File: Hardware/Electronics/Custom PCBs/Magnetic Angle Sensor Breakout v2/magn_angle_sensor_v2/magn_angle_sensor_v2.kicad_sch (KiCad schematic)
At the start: 57 parts, among them J1 JST PH 01x04, J2 USB C Receptacle, J3 120TR, U1 MT6701-CT, U2 RP2040, U2 W25Q128JVS, U4 SE8650X2-HF, U5 SN65HVD1050D, U6 XC6206P332MR, Y1 12MHz/12pF/50Ω/20ppm

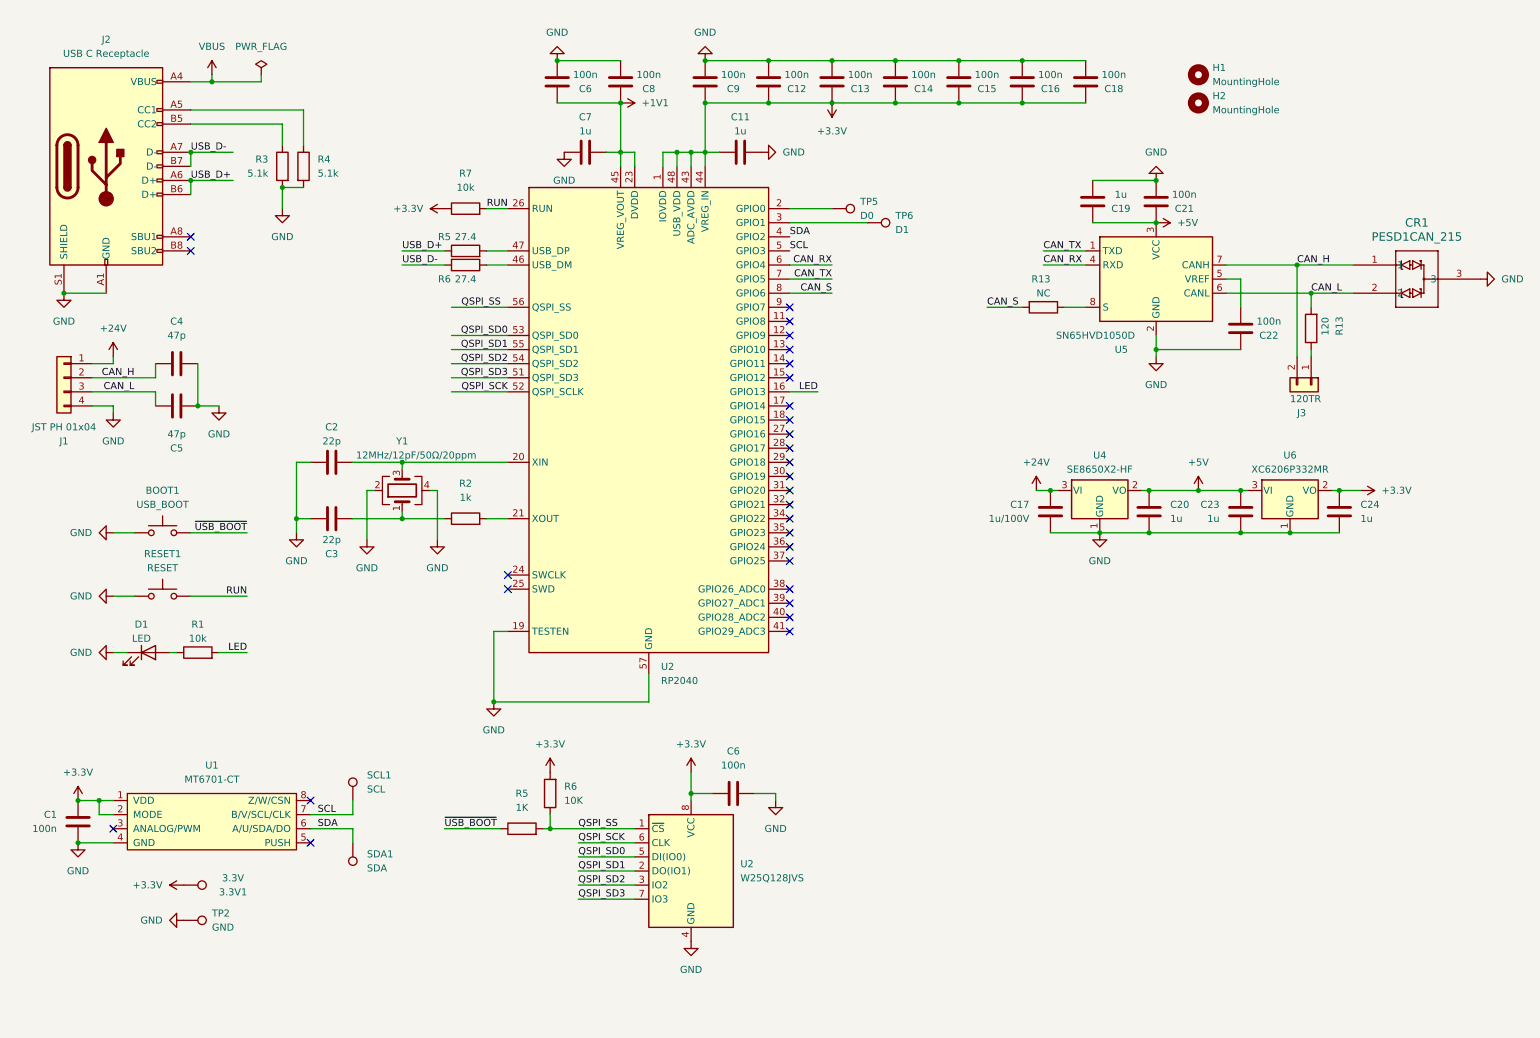
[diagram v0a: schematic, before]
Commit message: Finish CAN Magnetic Angle Sensor v2
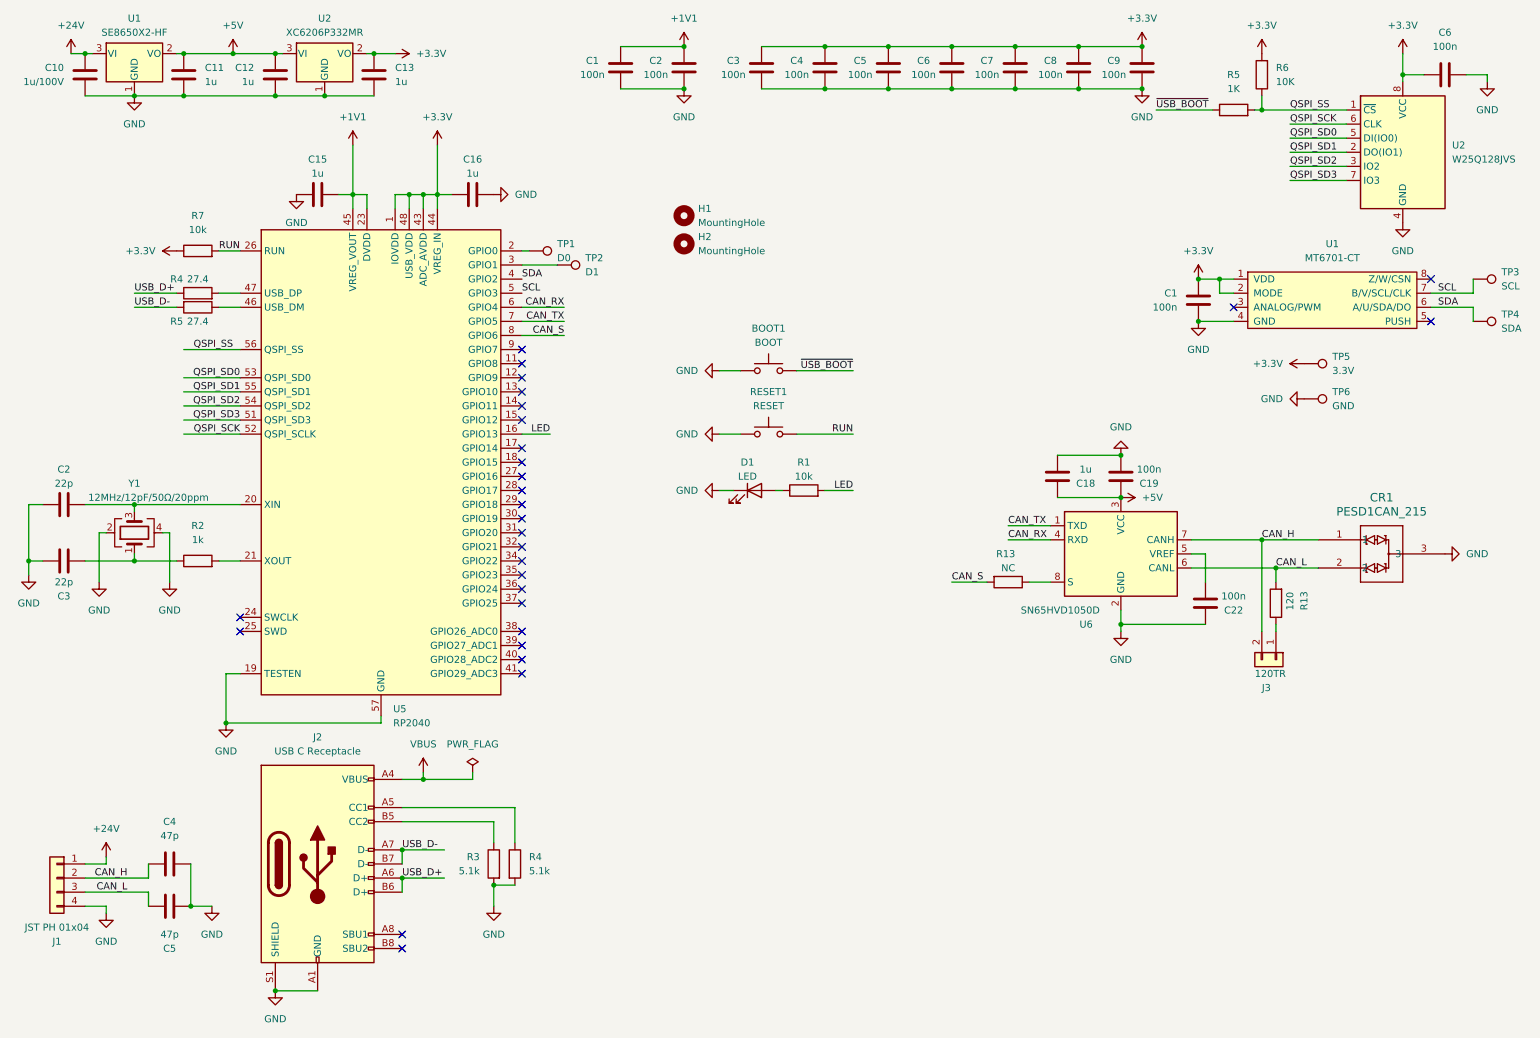
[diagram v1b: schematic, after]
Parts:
- removed 3.3V1: 3.3V, TestPoint:TestPoint_Pad_D1.0mm, symbol Connector:TestPoint
- removed C1, C14, C21, C6 (x2): 100n, Capacitor_SMD:C_0402_1005Metric, symbol Device:C
- removed C17: 1u/100V, Capacitor_SMD:C_0805_2012Metric, symbol Device:C
- removed C2, C3: 22p, Capacitor_SMD:C_0402_1005Metric, symbol Device:C
- removed C20, C23, C24: 1u, Capacitor_SMD:C_0402_1005Metric, symbol Device:C
- removed C4, C5: 47p, Capacitor_SMD:C_0402_1005Metric, symbol Device:C
- removed R13: 120, Resistor_SMD:R_0402_1005Metric, symbol Device:R
- removed R13: NC, Resistor_SMD:R_0402_1005Metric, symbol Device:R
- removed R4: 5.1k, Resistor_SMD:R_0402_1005Metric, symbol Device:R
- removed R5, R6: 27.4, Resistor_SMD:R_0402_1005Metric, symbol Device:R
- removed R5: 1K, Resistor_SMD:R_0402_1005Metric, symbol Device:R
- removed R6: 10K, Resistor_SMD:R_0402_1005Metric, symbol Device:R
- removed SCL1: SCL, TestPoint:TestPoint_Pad_D1.0mm, symbol Connector:TestPoint
- removed SDA1: SDA, TestPoint:TestPoint_Pad_D1.0mm, symbol Connector:TestPoint
- removed U2: RP2040, Package_DFN_QFN:QFN-56-1EP_7x7mm_P0.4mm_EP3.2x3.2mm, symbol MCU_RaspberryPi:RP2040
- removed U4: SE8650X2-HF, Package_TO_SOT_SMD:SOT-23, symbol Regulator_Linear:LF15_TO220
- removed U5: SN65HVD1050D, Package_SO:SOIC-8_3.9x4.9mm_P1.27mm, symbol Interface_CAN_LIN:SN65HVD1050D
- removed U6: XC6206P332MR, Package_TO_SOT_SMD:SOT-23, symbol Regulator_Linear:LF15_TO220
- added C1 (x2), C2, C3, C4, C5, C6 (x2): 100n, Capacitor_SMD:C_0402_1005Metric, symbol Device:C
- added C10: 1u/100V, Capacitor_SMD:C_0805_2012Metric, symbol Device:C
- added C2, C3: 22p, Capacitor_SMD:C_0402_1005Metric, symbol Device:C
- added C4, C5: 47p, Capacitor_SMD:C_0402_1005Metric, symbol Device:C
- added R13: NC, Resistor_SMD:R_0402_1005Metric, symbol Device:R
- added R13: 120, Resistor_SMD:R_0402_1005Metric, symbol Device:R
- added R4: 5.1k, Resistor_SMD:R_0402_1005Metric, symbol Device:R
- added R4, R5: 27.4, Resistor_SMD:R_0402_1005Metric, symbol Device:R
- added R5: 1K, Resistor_SMD:R_0402_1005Metric, symbol Device:R
- added R6: 10K, Resistor_SMD:R_0402_1005Metric, symbol Device:R
- added TP1: D0, TestPoint:TestPoint_Pad_D1.0mm, symbol Connector:TestPoint
- added TP3: SCL, TestPoint:TestPoint_Pad_D1.0mm, symbol Connector:TestPoint
- added TP4: SDA, TestPoint:TestPoint_Pad_D1.0mm, symbol Connector:TestPoint
- added U1: SE8650X2-HF, Package_TO_SOT_SMD:SOT-23, symbol Regulator_Linear:LF15_TO220
- added U2: XC6206P332MR, Package_TO_SOT_SMD:SOT-23, symbol Regulator_Linear:LF15_TO220
- added U5: RP2040, Package_DFN_QFN:QFN-56-1EP_7x7mm_P0.4mm_EP3.2x3.2mm, symbol MCU_RaspberryPi:RP2040
- added U6: SN65HVD1050D, Package_SO:SOIC-8_3.9x4.9mm_P1.27mm, symbol Interface_CAN_LIN:SN65HVD1050D
- BOOT1: value USB_BOOT -> BOOT
- C12, C13, C15, C16, C18: value 100n -> 1u
- C19, C7: value 1u -> 100n
- TP2: value GND -> D1
- TP5: value D0 -> 3.3V
- TP6: value D1 -> GND
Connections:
- net +1V1: now also C15.2, C1.2, C2.2, U5.23 (DVDD), U5.45 (VREG_VOUT), U5.50 (DVDD); no longer C7.2, C8.2
- net +24V: now also C10.2, U1.3 (VI)
- net +3.3V: now also C13.1, C16.1, C7.2, C8.2, TP5.1, C1.1, C3.2, C4.2, C5.2, C6.1, C6.2, R6.2, U2.2 (VO), U5.1 (IOVDD), U5.10 (IOVDD), U5.22 (IOVDD), U5.33 (IOVDD), U5.42 (IOVDD), U5.43 (ADC_AVDD), U5.44 (VREG_IN), U5.48 (USB_VDD), U5.49 (IOVDD); no longer C11.1, C12.2, C13.2, C15.2, C16.2, C18.2
- net +5V: now also C11.1, C12.1, C18.2, U1.2 (VO), U2.3 (VI), U6.3 (VCC)
- net CAN_H: now also C4.1, U6.7 (CANH)
- net CAN_L: now also C5.1, R13.2, U6.6 (CANL)
- net CAN_RX: now also U5.6 (GPIO4), U6.4 (RXD)
- net CAN_S: now also R13.2, U5.8 (GPIO6)
- net CAN_TX: now also U5.7 (GPIO5), U6.1 (TXD)
- net GND: now also C12.2, C13.2, C16.2, TP6.1, C1.1, C1.2, C10.1, C2.1, C2.1, C3.1, C3.1, C4.1, C4.2, C5.1, C5.2, C6.1, C6.2, R4.2, U1.1 (GND), U2.1 (GND), U5.19 (TESTEN), U5.57 (GND), U6.2 (GND); no longer C12.1, C13.1, C16.1, TP2.1
- net LED: now also U5.16 (GPIO13)
- net QSPI_SCK: now also U5.52 (QSPI_SCLK)
- net QSPI_SD0: now also U5.53 (QSPI_SD0)
- net QSPI_SD1: now also U5.55 (QSPI_SD1)
- net QSPI_SD2: now also U5.54 (QSPI_SD2)
- net QSPI_SD3: now also U5.51 (QSPI_SD3)
- net QSPI_SS: now also R5.2, R6.1, U5.56 (QSPI_SS)
- net RUN: now also U5.26 (RUN)
- net SCL: now also TP3.1, U5.5 (GPIO3)
- net SDA: now also TP4.1, U5.4 (GPIO2)
- net USB_D+: now also R4.1
- net USB_D-: now also R5.2
- net ~{USB_BOOT}: now also R5.1
- net at J3.1 (Pin_1): now also R13.1
- net at C22.1: now also U6.5 (VREF)
- net at J2.A5 (CC1): now also R4.1
- net at R2.1, Y1.1: now also C3.2
- net at R2.2: now also U5.21 (XOUT)
- net at Y1.3: now also C2.2, U5.20 (XIN)
- new net: R13.1, U6.8 (S)
- new net: TP1.1, U5.2 (GPIO0)
- new net: R5.1, U5.46 (USB_DM)
- new net: TP2.1, U5.3 (GPIO1)
- new net: R4.2, U5.47 (USB_DP)
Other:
- moved on the sheet: H1, H2
